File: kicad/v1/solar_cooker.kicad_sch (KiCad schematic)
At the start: 10 parts, among them SW1 SW_DPST_x2, U1 ATmega2560-16A, U2 microSD, U3 clock_module, U4 e-Paper, U5 anemometer, U6 BME680, U7 PT100, U8 GPS

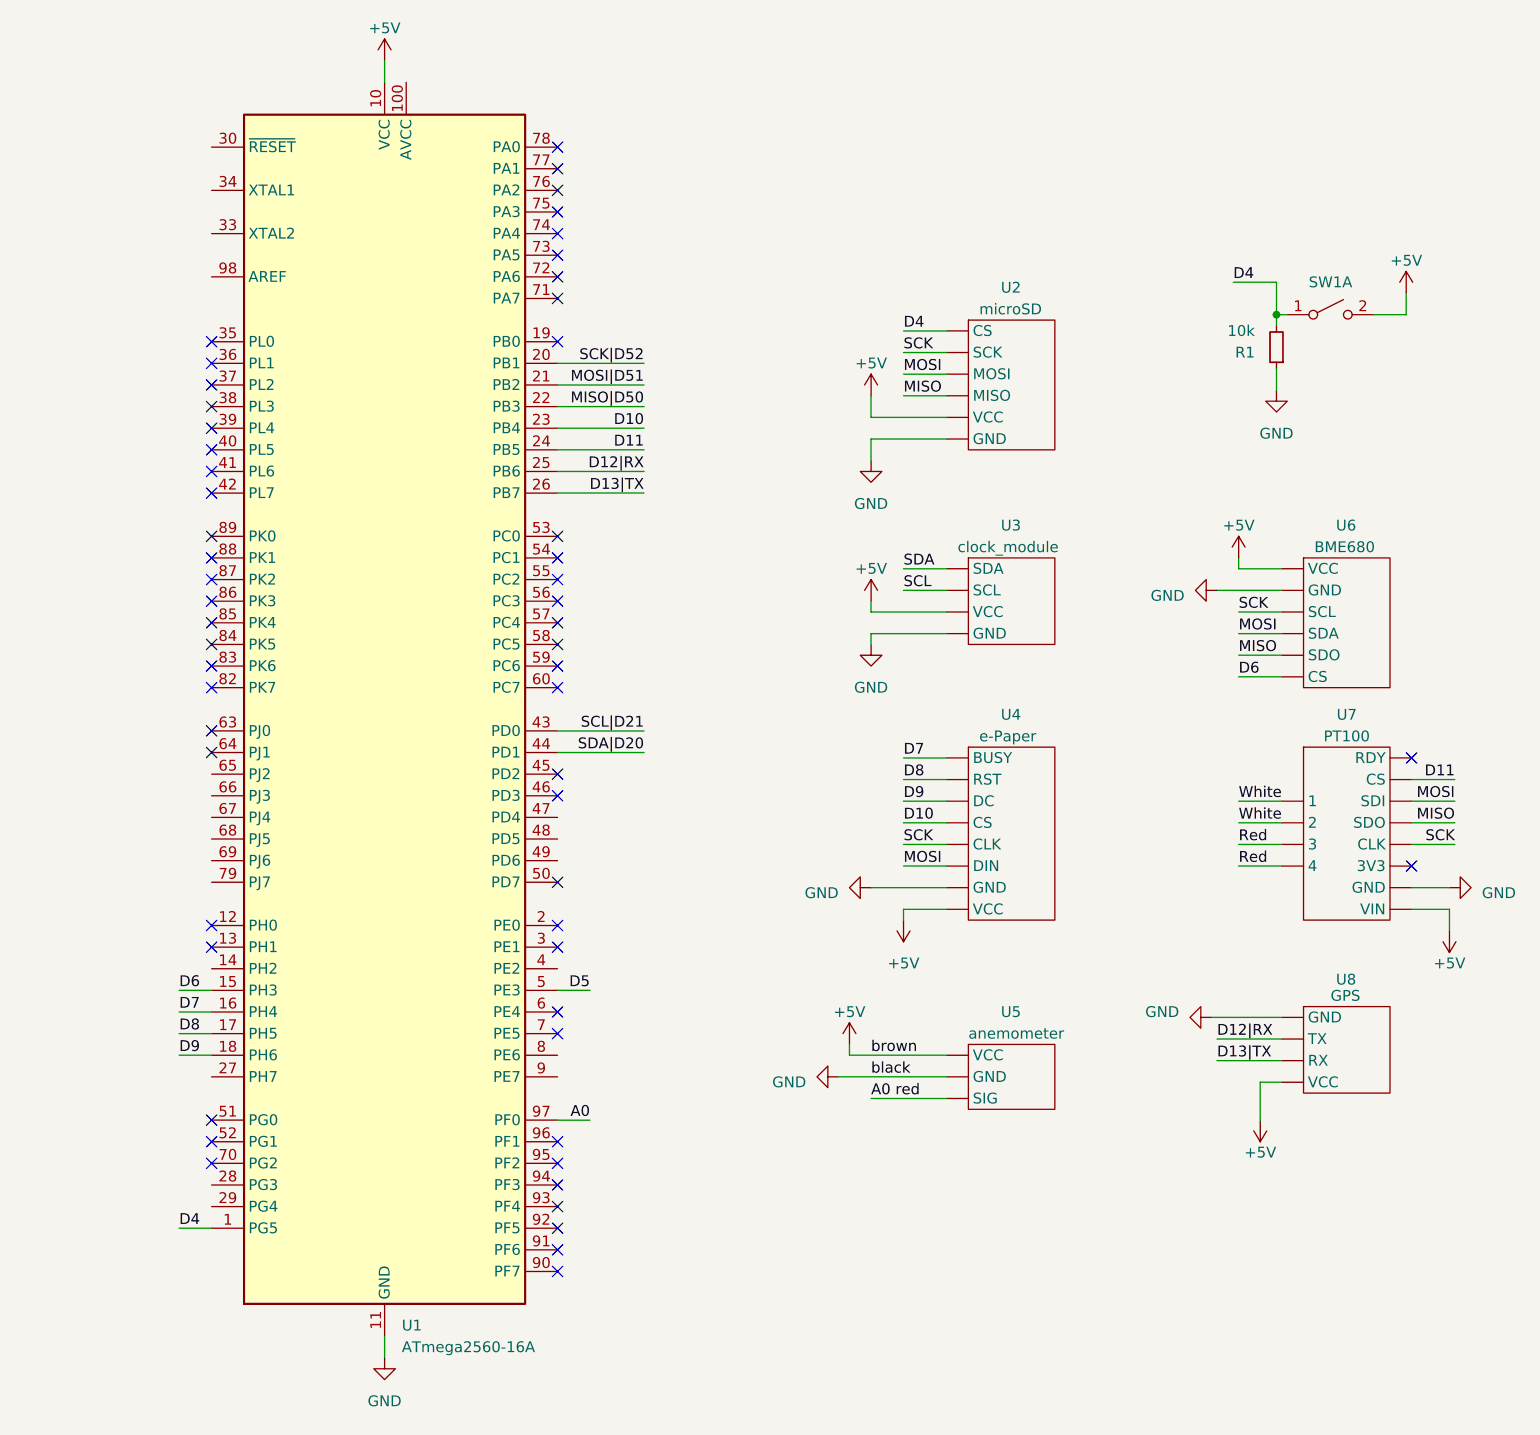
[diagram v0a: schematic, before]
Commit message: KiCad v2 update
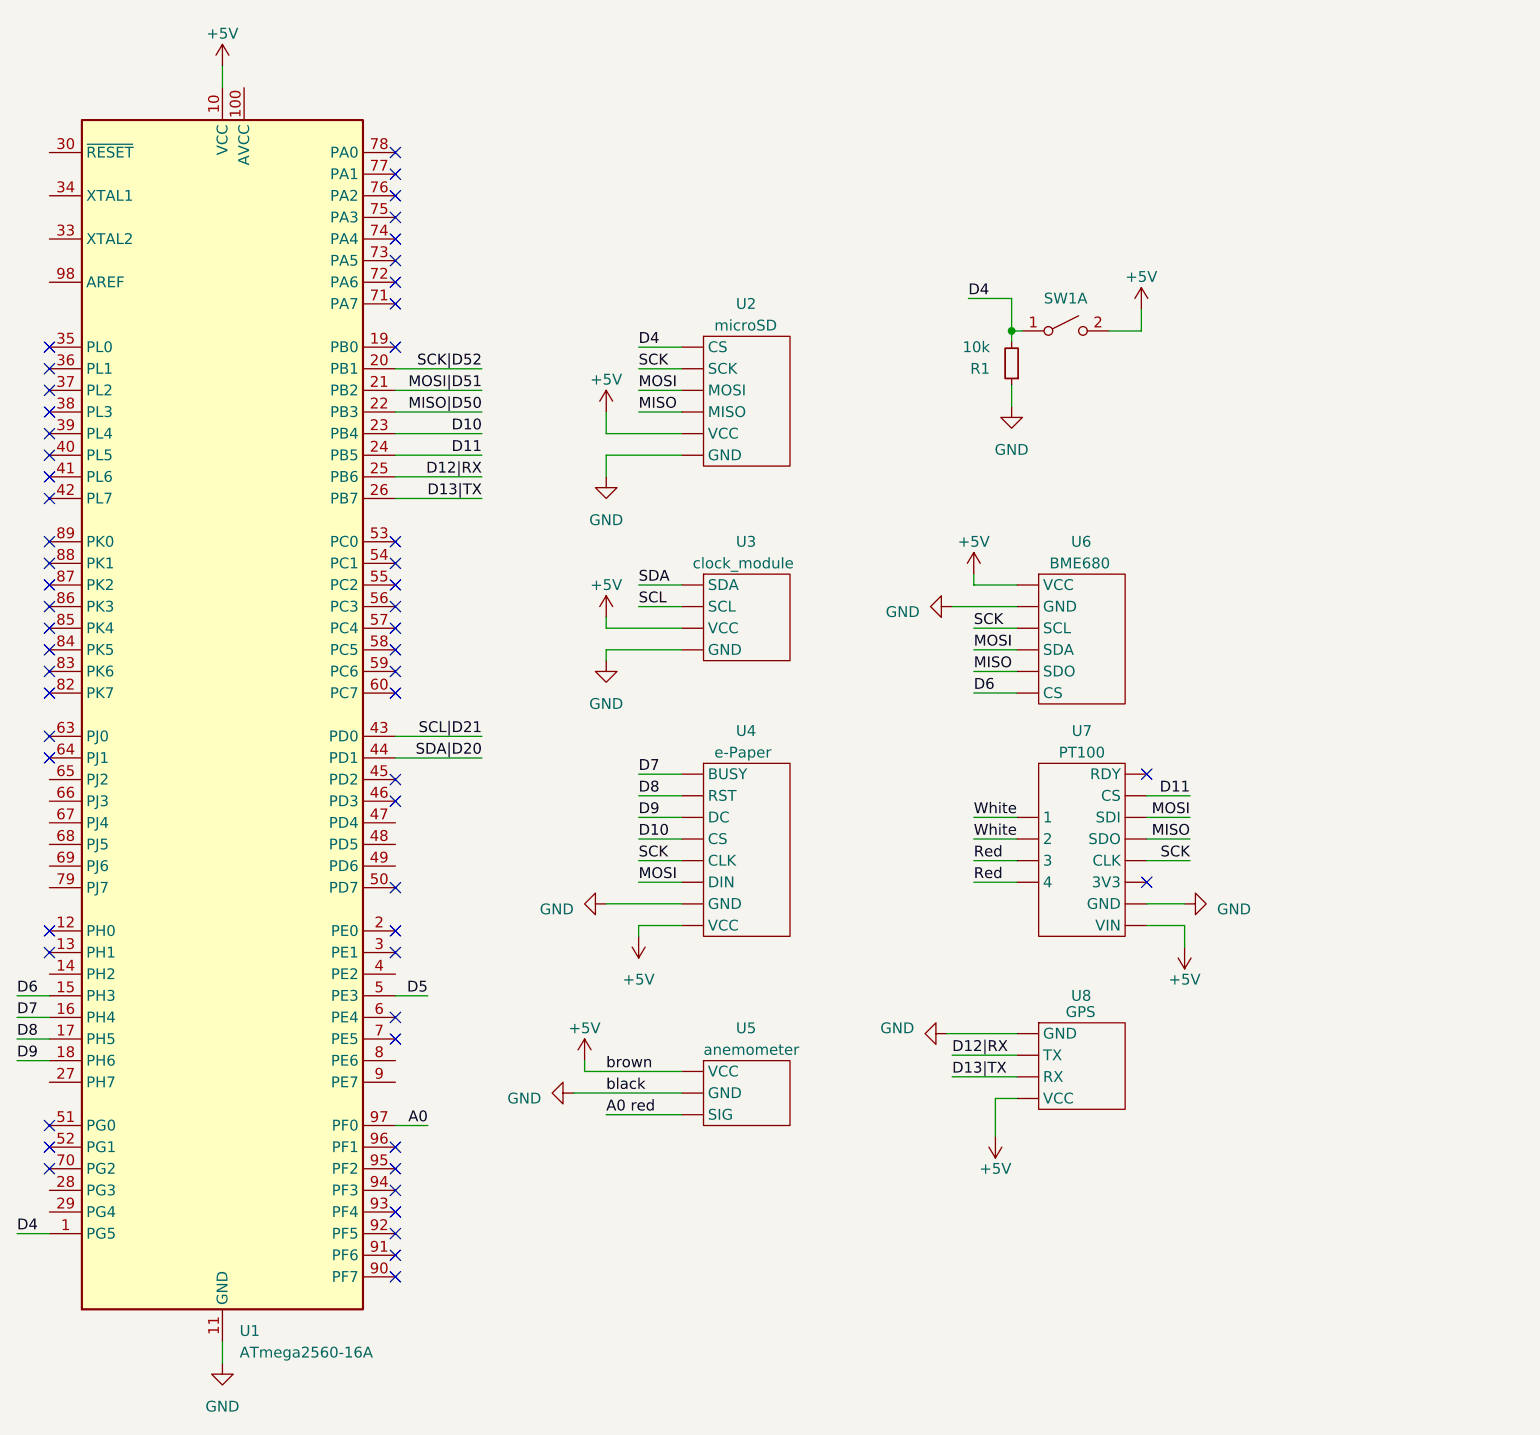
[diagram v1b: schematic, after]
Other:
- moved on the sheet: R1, SW1A, U1, U2, U3, U4, U5, U6, U7, U8
